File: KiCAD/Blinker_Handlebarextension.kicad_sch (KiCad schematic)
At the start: 4 parts, among them IC7 IS32LT3183A-GRLA3-TR, SW2 RotaryEncoder_Switch

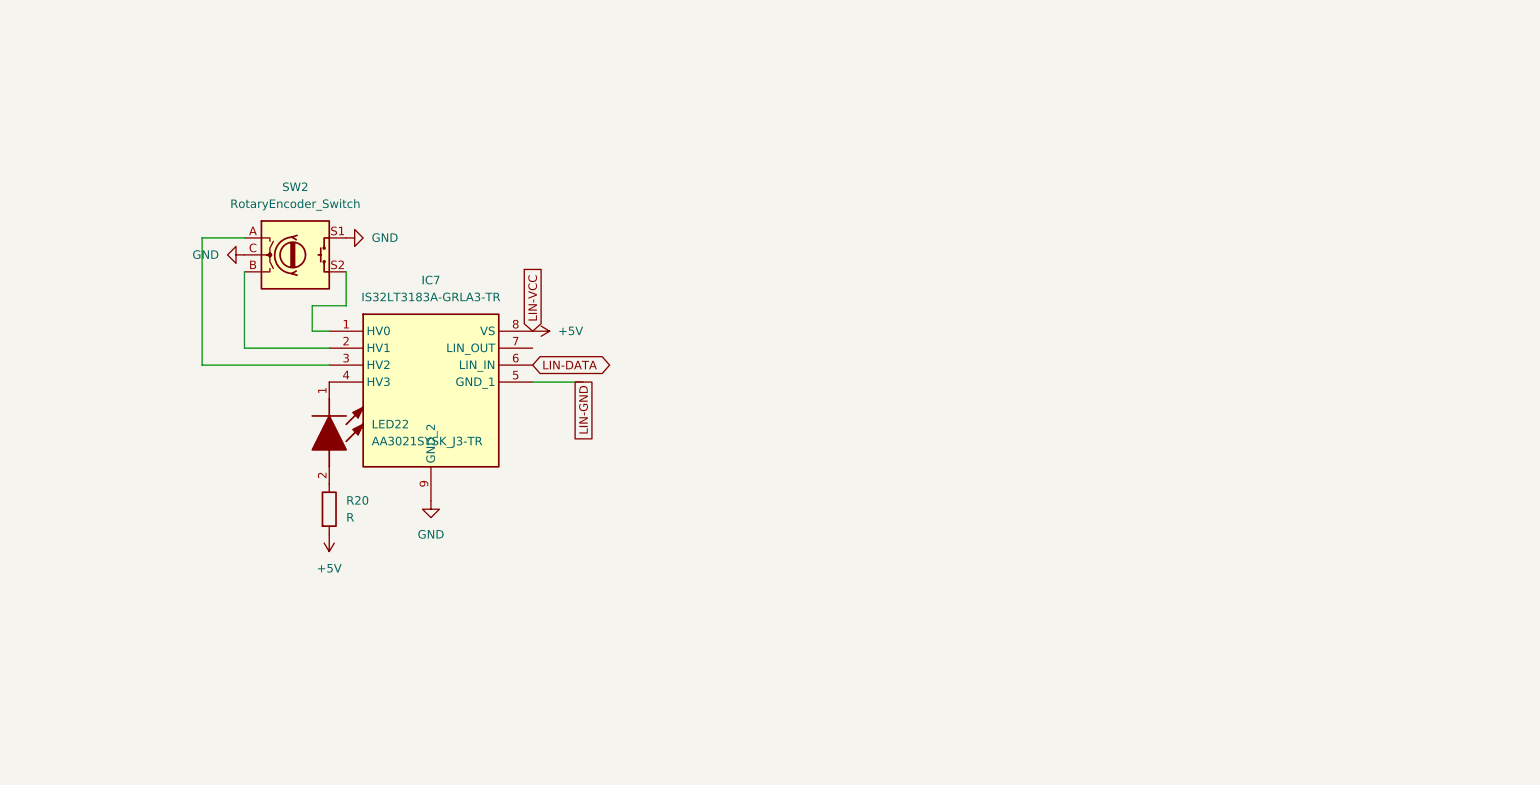
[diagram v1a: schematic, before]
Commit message: update
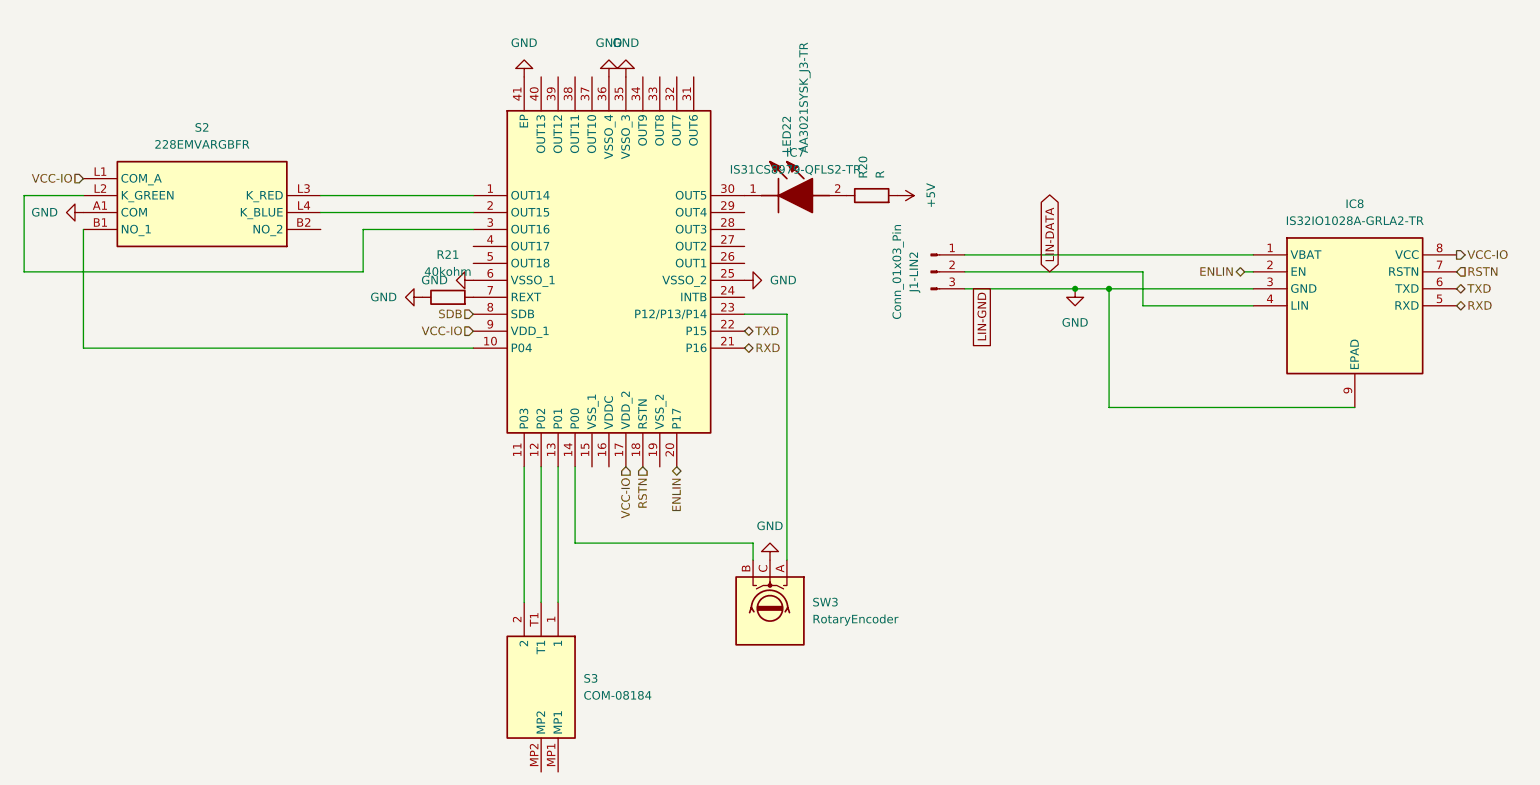
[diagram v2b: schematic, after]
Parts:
- removed IC7: IS32LT3183A-GRLA3-TR, SOIC127P600X170-9N, symbol SamacSys_Parts:IS32LT3183A-GRLA3-TR
- removed SW2: RotaryEncoder_Switch, symbol Device:RotaryEncoder_Switch
- added IC7: IS31CS8979-QFLS2-TR, QFN50P600X600X80-41N-D, symbol SamacSys_Parts:IS31CS8979-QFLS2-TR
- added IC8: IS32IO1028A-GRLA2-TR, SOIC127P600X170-9N, symbol SamacSys_Parts:IS32IO1028A-GRLA2-TR
- added J1-LIN2: Conn_01x03_Pin, symbol Connector:Conn_01x03_Pin
- added R21: 40kohm, symbol Device:R
- added S2: 228EMVARGBFR, 228EMVARGBFR, symbol SamacSys_Parts:228EMVARGBFR
- added S3: COM-08184, COM08184, symbol SamacSys_Parts:COM-08184
- added SW3: RotaryEncoder, symbol Device:RotaryEncoder
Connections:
- net GND: now also IC7.25 (VSSO_2), IC7.35 (VSSO_3), IC7.36 (VSSO_4), IC7.41 (EP), IC7.6 (VSSO_1), IC8.3 (GND), IC8.9 (EPAD), J1-LIN2.3 (Pin_3), R21.1, S2.A1 (COM), SW3.C
- net LIN-DATA: now also IC8.4 (LIN), J1-LIN2.2 (Pin_2)
- net at LED22.1 (K): now also IC7.30 (OUT5)
- new net: IC7.10 (P04), S2.B1 (NO_1)
- new net: IC7.3 (OUT16), S2.L2 (K_GREEN)
- new net: IC7.1 (OUT14), S2.L3 (K_RED)
- new net: IC7.2 (OUT15), S2.L4 (K_BLUE)
- new net: IC8.1 (VBAT), J1-LIN2.1 (Pin_1)
- new net: IC7.13 (P01), S3.1
- new net: IC7.11 (P03), S3.2
- new net: IC7.12 (P02), S3.T1
- new net: IC7.7 (REXT), R21.2
- new net: IC7.23 (P12/P13/P14), SW3.A
- new net: IC7.14 (P00), SW3.B
- new net ENLIN: IC7.20 (P17), IC8.2 (EN)
- new net RSTN: IC7.18 (RSTN), IC8.7 (RSTN)
- new net RXD: IC7.21 (P16), IC8.5 (RXD)
- new net SDB: IC7.8 (SDB)
- new net TXD: IC7.22 (P15), IC8.6 (TXD)
- new net VCC-IO: IC7.17 (VDD_2), IC7.9 (VDD_1), IC8.8 (VCC), S2.L1 (COM_A)
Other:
- moved on the sheet: LED22, R20
